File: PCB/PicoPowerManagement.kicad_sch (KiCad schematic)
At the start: 39 parts, among them J10 UART Header, J11 ATX 24P Connection, J2 DEBUG, J3 DisplayPowerSwitch, J4 Pi1PowerSwitch, J5 Pi2PowerSwitch, J6 Pi4PowerSwitch, J7 NAS Fan 1, J8 NAS Fan 2, J9 Pi3PowerSwitch, Q1 2N3904, Q14 NMOS, Q15 NMOS, Q2 PMOS, Q3 PMOS, SW1 Power, U1 LSF0101DRYR, U13 LM338T, U14 LM338T, U2 LSF0101DRYR, U6 FUSB302MPX, U7 FUSB302MPX, U8 FUSB302MPX

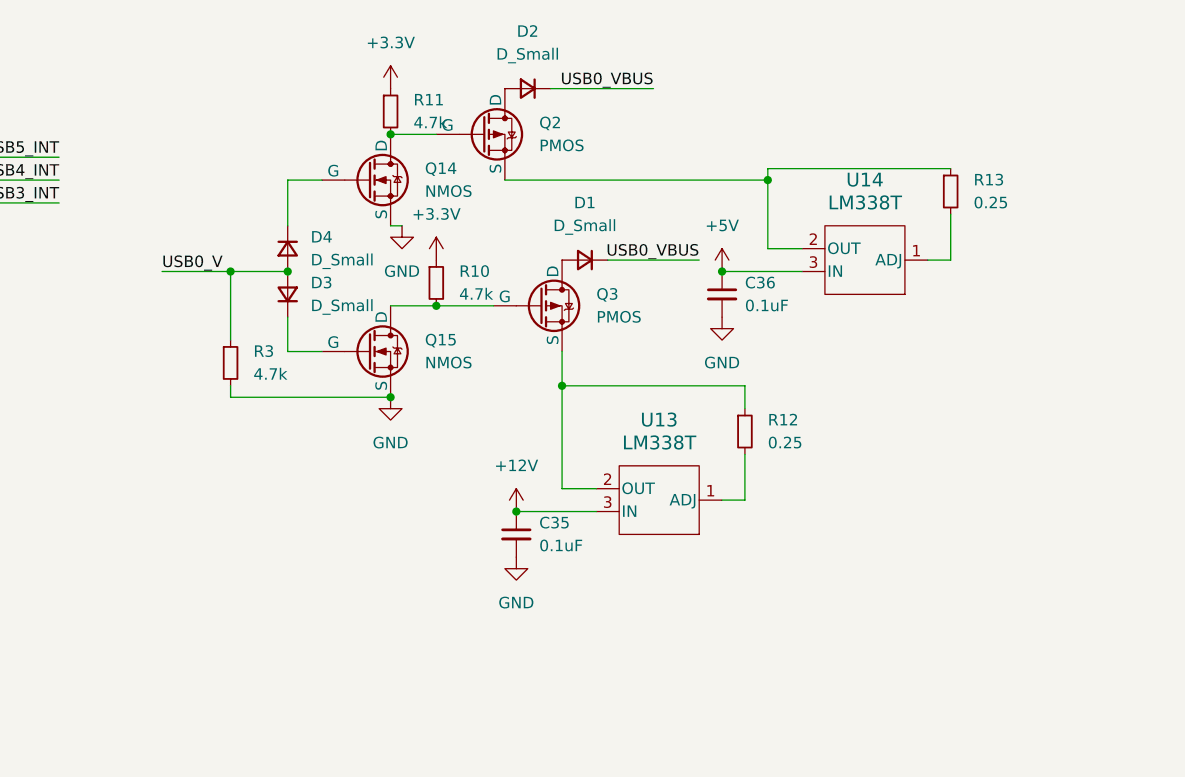
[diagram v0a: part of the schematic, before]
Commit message: No code changes made.
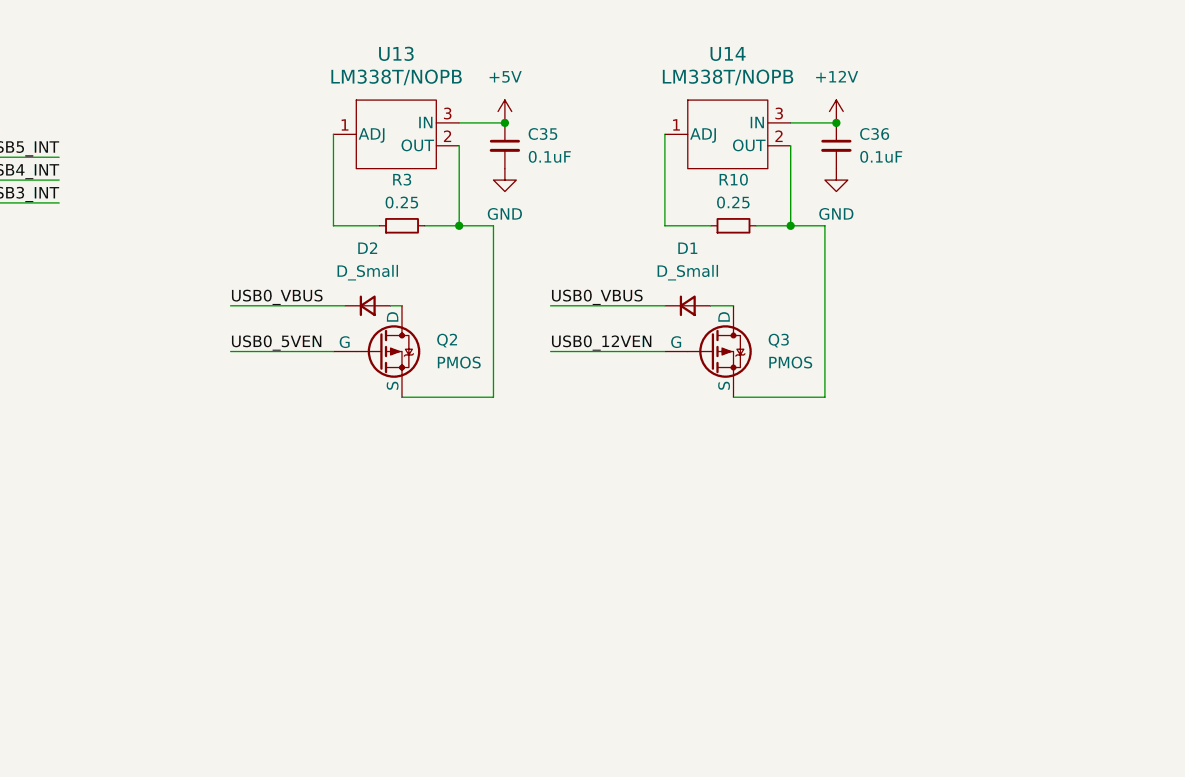
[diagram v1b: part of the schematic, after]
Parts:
- removed D3, D4: D_Small, symbol Device:D_Small
- removed Q14, Q15: NMOS, symbol Simulation_SPICE:NMOS
- removed R11: 4.7k, symbol Device:R_Small
- removed R12, R13: 0.25, symbol Device:R_Small
- R10, R3: value 4.7k -> 0.25
- U13, U14: value LM338T -> LM338T/NOPB
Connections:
- net +12V: now also C36.1, U14.3 (IN); no longer C35.1, U13.3 (IN)
- net +3.3V: no longer R10.1
- net +5V: now also C35.1, U13.3 (IN); no longer C36.1, U14.3 (IN)
- net GND: no longer R3.2
- net USB0_V: no longer R3.1
- net at U14.1 (ADJ): now also R10.1
- net at Q2.3 (S): now also R3.2, U13.2 (OUT); no longer U14.2 (OUT)
- net USB0_5VEN: now reaches Q2.2 (G)
- net at Q3.3 (S): now also R10.2, U14.2 (OUT); no longer U13.2 (OUT)
- net at U13.1 (ADJ): now also R3.1
- net USB0_12VEN: now reaches Q3.2 (G)
- net USB0_12VEN: no longer R10.2
